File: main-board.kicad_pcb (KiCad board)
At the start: 4 copper layers, 10.4 x 12.3 mm, 9 parts, among them IC1 FS312F-G, J1 BAT-, J2 POS_OUT, J3 BAT_POS, J4 -, Q1 FS8205A

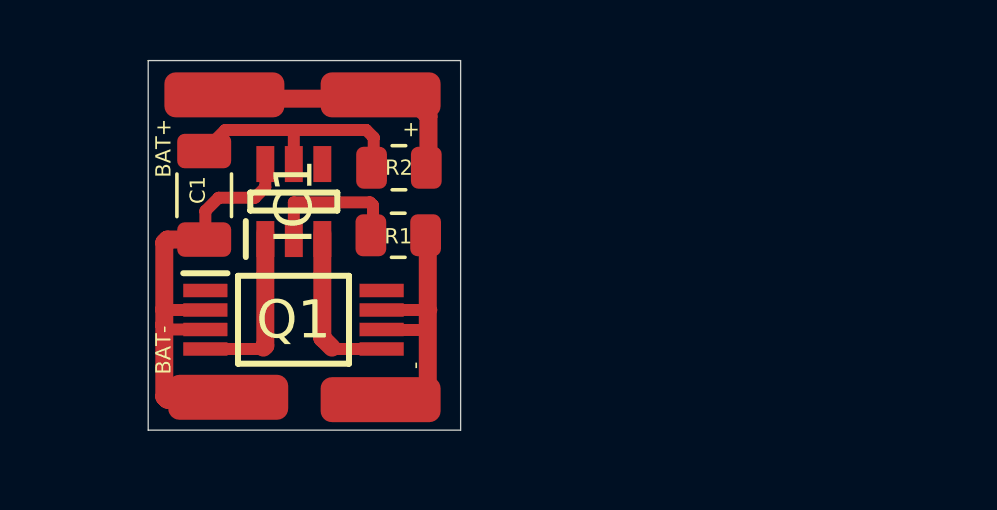
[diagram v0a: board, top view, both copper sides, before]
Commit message: minor
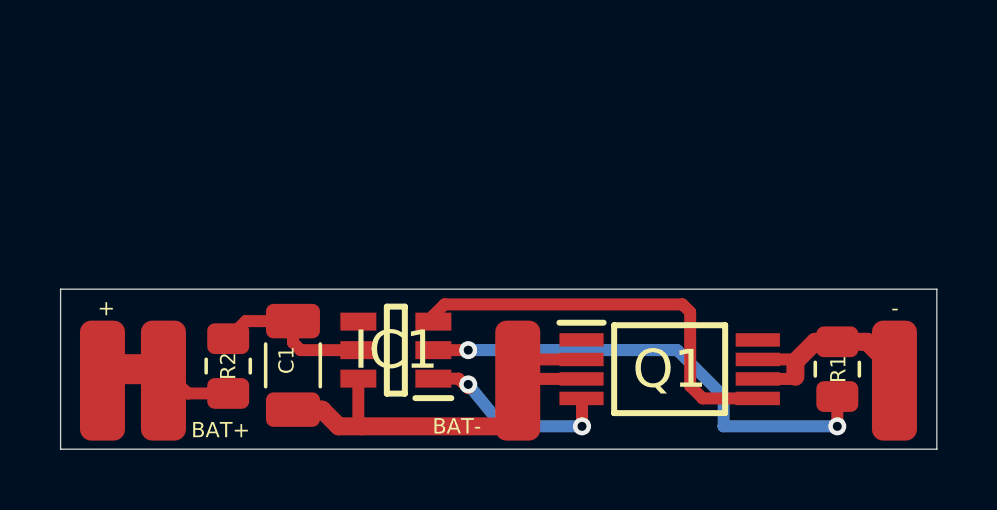
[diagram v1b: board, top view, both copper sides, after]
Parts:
- moved J4 17.1 mm to (158.0, 96.6), turned to 180 degrees
- moved R1 15.3 mm to (156.1, 96.3), turned to -90 degrees
- moved J2 13.3 mm to (131.6, 96.6), turned to 180 degrees
- moved Q1 12.6 mm to (150.5, 96.3)
- moved J3 9.74 mm to (133.6, 96.6), turned to 180 degrees
- moved J1 9.67 mm to (145.4, 96.6), turned to 180 degrees
- moved R2 8.72 mm to (135.8, 96.2), turned to -90 degrees
- moved C1 6.40 mm to (137.9, 96.1)
- moved IC1 6.01 mm to (141.4, 95.6), turned to 180 degrees
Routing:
- net Net-(IC1-Pad2): track 4.88 -> 16.1 mm, vias 0 -> 2
- net Net-(IC1-Pad3): track 5.64 -> 13.9 mm
- net BAT_POS: track 9.38 -> 4.53 mm
- net Net-(C1-Pad2): track 8.17 -> 5.40 mm
- net BAT_NEG: track 15.3 -> 13.2 mm
- net Net-(J4-Pad1): track 8.89 -> 7.03 mm
- net Net-(IC1-Pad1): track 5.81 -> 6.81 mm, vias 0 -> 2
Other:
- board size 10.4 x 12.3 mm -> 29.2 x 5.3 mm
